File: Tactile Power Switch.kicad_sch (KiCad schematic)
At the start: 15 parts, among them J1 OSTTC020162, J2 OSTTC020162, Q1 BC847B_215, Q2 BC847B_215, Q4 NDT2955, SW1 SW_SPST

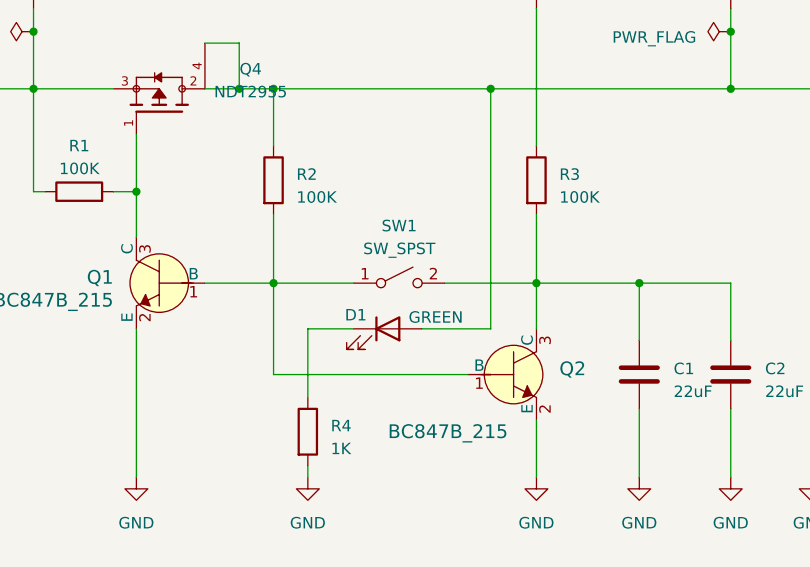
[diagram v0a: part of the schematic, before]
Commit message: mfg file initiated
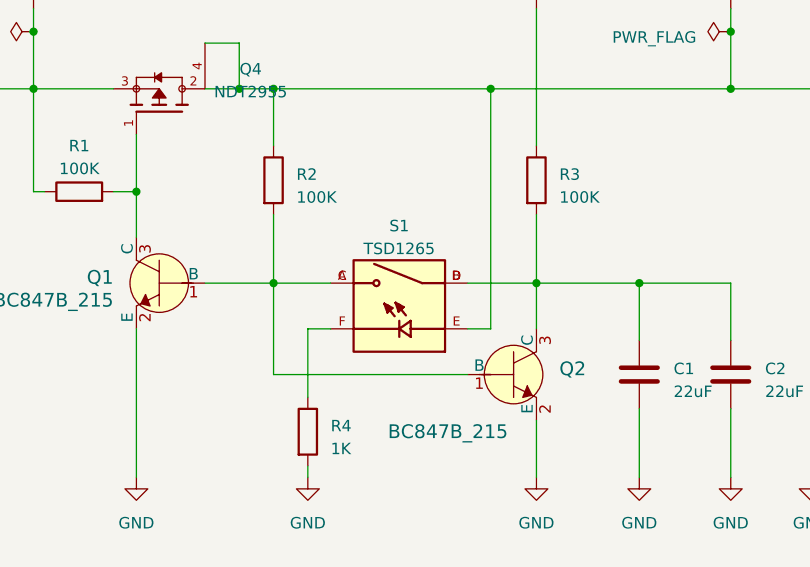
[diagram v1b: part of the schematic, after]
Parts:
- removed D1: GREEN, LED_SMD:LED_0603_1608Metric, symbol Device:LED
- removed SW1: SW_SPST, Button_Switch_SMD:SW_SPST_TL3342, symbol Switch:SW_SPST
- added S1: TSD1265, SW_TSD1265:SW_TSD1265, symbol TSD1265:TSD1265
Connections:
- net VDD: now also S1.E
- net at Q1.1 (B), Q2.1 (B), R2.2: now also S1.A, S1.C
- net at C1.1, C2.1, Q2.3 (C)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: now also S1.B, S1.D
- net at R4.1: now also S1.F
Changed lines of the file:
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@@
 	(wire
 		(pts
-			(xy 153.67 97.79) (xy 146.05 97.79)
+			(xy 153.67 97.79) (xy 151.13 97.79)
 		)
 		(stroke
@@
 	(wire
 		(pts
-			(xy 148.59 92.71) (xy 158.75 92.71)
+			(xy 151.13 92.71) (xy 158.75 92.71)
 		)
 		(stroke
@@
 	(wire
 		(pts
-			(xy 129.54 92.71) (xy 138.43 92.71)
+			(xy 129.54 92.71) (xy 135.89 92.71)
 		)
 		(stroke
@@
 	(wire
 		(pts
-			(xy 133.35 97.79) (xy 138.43 97.79)
+			(xy 133.35 97.79) (xy 135.89 97.79)
 		)
 		(stroke
@@
 	)
 	(symbol
-		(lib_id "Switch:SW_SPST")
-		(at 143.51 92.71 0)
+		(lib_id "TSD1265:TSD1265")
+		(at 143.51 95.25 0)
+		(mirror y)
 		(unit 1)
 		(exclude_from_sim no)
@@
 		(on_board yes)
 		(dnp no)
-		(fields_autoplaced yes)
-		(property "Reference" "SW1"
+		(property "Reference" "S1"
 			(at 143.51 86.36 0)
 			(effects
@@
 			)
 		)
-		(property "Value" "SW_SPST"
+		(property "Value" "TSD1265"
 			(at 143.51 88.9 0)
 			(effects
@@
 			)
 		)
-		(property "Footprint" "Button_Switch_SMD:SW_SPST_TL3342"
-			(at 143.51 92.71 0)
-			(effects
-				(font
-					(size 1.27 1.27)
-				)
-				(hide yes)
-			)
-		)
-		(property "Datasheet" "~"
-			(at 143.51 92.71 0)
-			(effects
-				(font
-					(size 1.27 1.27)
-				)
-				(hide yes)
-			)
-		)
-		(property "Description" "Single Pole Single Throw (SPST) switch"
-			(at 143.51 92.71 0)
-			(effects
-				(font
-					(size 1.27 1.27)
-				)
-				(hide yes)
-			)
-		)
-		(pin "1"
-		)
-		(pin "2"
+		(property "Footprint" "SW_TSD1265:SW_TSD1265"
+			(at 143.51 95.25 0)
+			(effects
+				(font
+					(size 1.27 1.27)
+				)
+				(justify bottom)
+				(hide yes)
+			)
+		)
+		(property "Datasheet" ""
+			(at 143.51 95.25 0)
+			(effects
+				(font
+					(size 1.27 1.27)
+				)
+				(hide yes)
+			)
+		)
+		(property "Description" "\nTactile Push Button Switch Momentary\n"
+			(at 143.51 95.25 0)
+			(effects
+				(font
+					(size 1.27 1.27)
+				)
+				(justify bottom)
+				(hide yes)
+			)
+		)
+		(property "MF" "Omten Electronics"
+			(at 143.51 95.25 0)
+			(effects
+				(font
+					(size 1.27 1.27)
+				)
+				(justify bottom)
+				(hide yes)
+			)
+		)
+		(property "MAXIMUM_PACKAGE_HEIGHT" "6.5 mm"
+			(at 143.51 95.25 0)
+			(effects
+				(font
+					(size 1.27 1.27)
+				)
+				(justify bottom)
+				(hide yes)
+			)
+		)
+		(property "Package" "Package"
+			(at 143.51 95.25 0)
+			(effects
+				(font
+					(size 1.27 1.27)
+				)
+				(justify bottom)
+				(hide yes)
+			)
+		)
+		(property "Price" "None"
+			(at 143.51 95.25 0)
+			(effects
+				(font
+					(size 1.27 1.27)
+				)
+				(justify bottom)
+				(hide yes)
+			)
+		)
+		(property "Check_prices" "https://www.snapeda.com/parts/TSD1265/Omten+Electronics/view-part/?ref=eda"
+			(at 143.51 95.25 0)
+			(effects
+				(font
+					(size 1.27 1.27)
+				)
+				(justify bottom)
+				(hide yes)
+			)
+		)
+		(property "STANDARD" "Manufacturer Recommendations"
+			(at 143.51 95.25 0)
+			(effects
+				(font
+					(size 1.27 1.27)
+				)
+				(justify bottom)
+				(hide yes)
+			)
+		)
+		(property "PARTREV" "N/A"
+			(at 143.51 95.25 0)
+			(effects
+				(font
+					(size 1.27 1.27)
+				)
+				(justify bottom)
+				(hide yes)
+			)
+		)
+		(property "SnapEDA_Link" "https://www.snapeda.com/parts/TSD1265/Omten+Electronics/view-part/?ref=snap"
+			(at 143.51 95.25 0)
+			(effects
+				(font
+					(size 1.27 1.27)
+				)
+				(justify bottom)
+				(hide yes)
+			)
+		)
+		(property "MP" "TSD1265"
+			(at 143.51 95.25 0)
+			(effects
+				(font
+					(size 1.27 1.27)
+				)
+				(justify bottom)
+				(hide yes)
+			)
+		)
+		(property "Availability" "Not in stock"
+			(at 143.51 95.25 0)
+			(effects
+				(font
+					(size 1.27 1.27)
+				)
+				(justify bottom)
+				(hide yes)
+			)
+		)
+		(property "MANUFACTURER" "Omten Electronics"
+			(at 143.51 95.25 0)
+			(effects
+				(font
+					(size 1.27 1.27)
+				)
+				(justify bottom)
+				(hide yes)
+			)
+		)
+		(pin "A"
+		)
+		(pin "B"
+		)
+		(pin "C"
+		)
+		(pin "D"
+		)
+		(pin "E"
+		)
+		(pin "F"
 		)
 		(instances
-			(project ""
+			(project "Tactile Power Switch"
 				(path "/72a9c836-61c4-4172-ab46-eebab5956cc2"
-					(reference "SW1")
+					(reference "S1")
 					(unit 1)
 				)
@@
 					(unit 1)
 				)
-			)
-		)
-	)
-	(symbol
-		(lib_id "Device:LED")
-		(at 142.24 97.79 0)
-		(unit 1)
-		(exclude_from_sim no)
-		(in_bom yes)
-		(on_board yes)
-		(dnp no)
-		(property "Reference" "D1"
-			(at 138.684 96.266 0)
-			(effects
-				(font
-					(size 1.27 1.27)
-				)
-			)
-		)
-		(property "Value" "GREEN"
-			(at 147.574 96.52 0)
-			(effects
-				(font
-					(size 1.27 1.27)
-				)
-			)
-		)
-		(property "Footprint" "LED_SMD:LED_0603_1608Metric"
-			(at 142.24 97.79 0)
-			(effects
-				(font
-					(size 1.27 1.27)
-				)
-				(hide yes)
-			)
-		)
-		(property "Datasheet" "~"
-			(at 142.24 97.79 0)
-			(effects
-				(font
-					(size 1.27 1.27)
-				)
-				(hide yes)
-			)
-		)
-		(property "Description" "Light emitting diode"
-			(at 142.24 97.79 0)
-			(effects
-				(font
-					(size 1.27 1.27)
-				)
-				(hide yes)
-			)
-		)
-		(pin "1"
-		)
-		(pin "2"
-		)
-		(instances
-			(project ""
-				(path "/72a9c836-61c4-4172-ab46-eebab5956cc2"
-					(reference "D1")
-					(unit 1)
-				)
